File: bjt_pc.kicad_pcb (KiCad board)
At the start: 2 copper layers, 130 x 79 mm, 72 parts, among them J1 Conn_02x10_Odd_Even

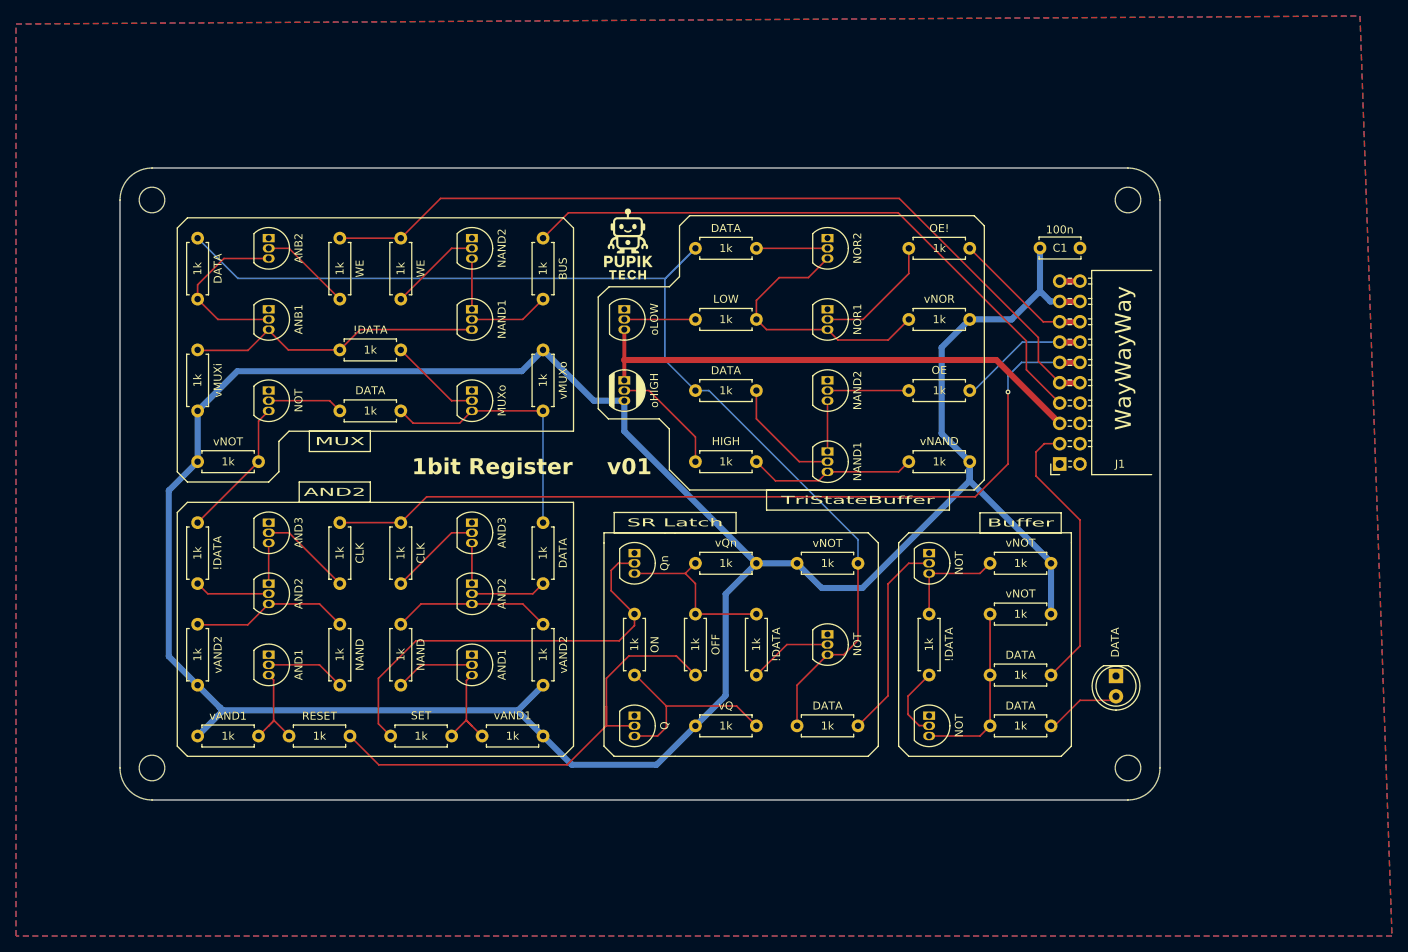
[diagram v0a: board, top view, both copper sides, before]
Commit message: Finalized compressed 1.0
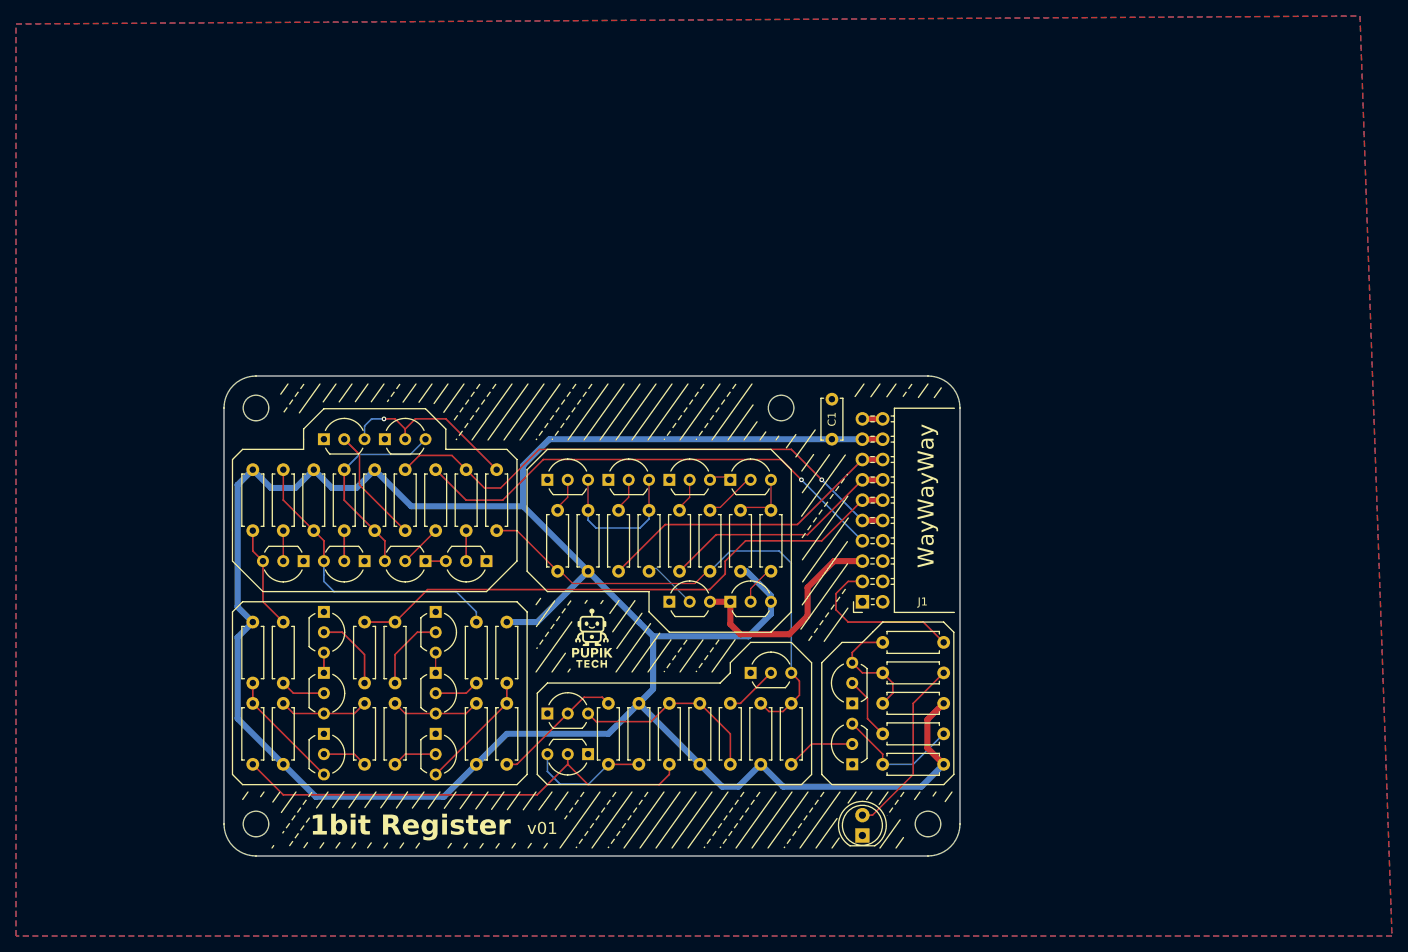
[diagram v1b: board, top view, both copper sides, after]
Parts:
- Qand11, Qand12, Qand13, Qand21, Qand22, Qand23, Qbuf1, Qbuf2, Qmux1, Qmux2, Qmux3, Qmux4, Qmux5, Qmux6, Qsrl1, Qsrl2, Qsrl3, Qtsb2, Qtsb3, Qtsb4, Qtsb5, Qtsb6: footprint Custom_Footprints:TO-92_Inline_disp -> Package_TO_SOT_THT:TO-92_Inline_Wide
- Qtsb1: footprint Custom_Footprints:TO-92_Inline_PNP_disp -> Package_TO_SOT_THT:TO-92_Inline_Wide
- moved R1 57.2 mm to (143.5, 105.4), turned to 90 degrees
- moved REF** 50.6 mm to (167.6, 85.0)
- moved G*** 49.4 mm to (144.0, 114.0)
- moved R4 48.9 mm to (147.3, 97.8), turned to -90 degrees
- moved Qtsb4 46.2 mm to (138.4, 94.0), turned to 0 degrees
- moved sDATA4 43.9 mm to (139.7, 105.4), turned to 90 degrees
- moved sDATA1 43.0 mm to (132.1, 92.7), turned to -90 degrees
- moved R5 42.7 mm to (154.9, 105.4), turned to 90 degrees
- moved Qmux4 40.4 mm to (130.8, 104.1), turned to 180 degrees
- moved D1 37.4 mm to (177.8, 138.4), turned to 90 degrees
- moved Qtsb2 37.0 mm to (153.7, 109.2), turned to 0 degrees
- moved C1 35.3 mm to (174.0, 88.9), turned to 90 degrees
- moved Qtsb3 34.7 mm to (146.1, 94.0), turned to 0 degrees
- moved R33 32.3 mm to (109.2, 92.7)
- moved Qmux3 32.0 mm to (123.2, 104.1), turned to 180 degrees
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- renumbered DATA to D1
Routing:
- net /DATA: track 142.5 -> 65.2 mm
- net /WE: track 105.9 -> 67.8 mm, vias 0 -> 1
- net Net-(Qsrl2-B): track 54.0 -> 16.5 mm
- net /BUSo: track 64.1 -> 28.2 mm
- net /CLK: track 107.3 -> 72.0 mm, vias 1 -> 0
- net /nOE: track 17.6 -> 38.8 mm
- net /VCC: track 326.0 -> 306.7 mm
- net /AlwaysOn: track 25.5 -> 8.67 mm
- net /BUSi: track 77.9 -> 61.2 mm, vias 0 -> 1
- net Net-(Qtsb3-C): track 34.6 -> 18.4 mm
- net /RAW: track 35.0 -> 21.1 mm
- net Net-(Qtsb5-C): track 21.0 -> 7.62 mm
- net /OE: track 16.8 -> 30.1 mm
- net /LED: track 9.65 -> 22.7 mm
- net Net-(Qmux3-C): track 37.5 -> 25.3 mm
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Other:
- board size 130 x 79 mm -> 92 x 60 mm
- board text removed: "AND2"
- board text removed: "Buffer"
- board text removed: "MUX"
- board text removed: "SR Latch"
- board text removed: "TriStateBuffer"
